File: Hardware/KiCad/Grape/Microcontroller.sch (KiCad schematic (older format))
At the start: 14 parts, among them J3 ARDUINO_R3, U4 ATMEGA328P_TQFP, Y1 16MHz

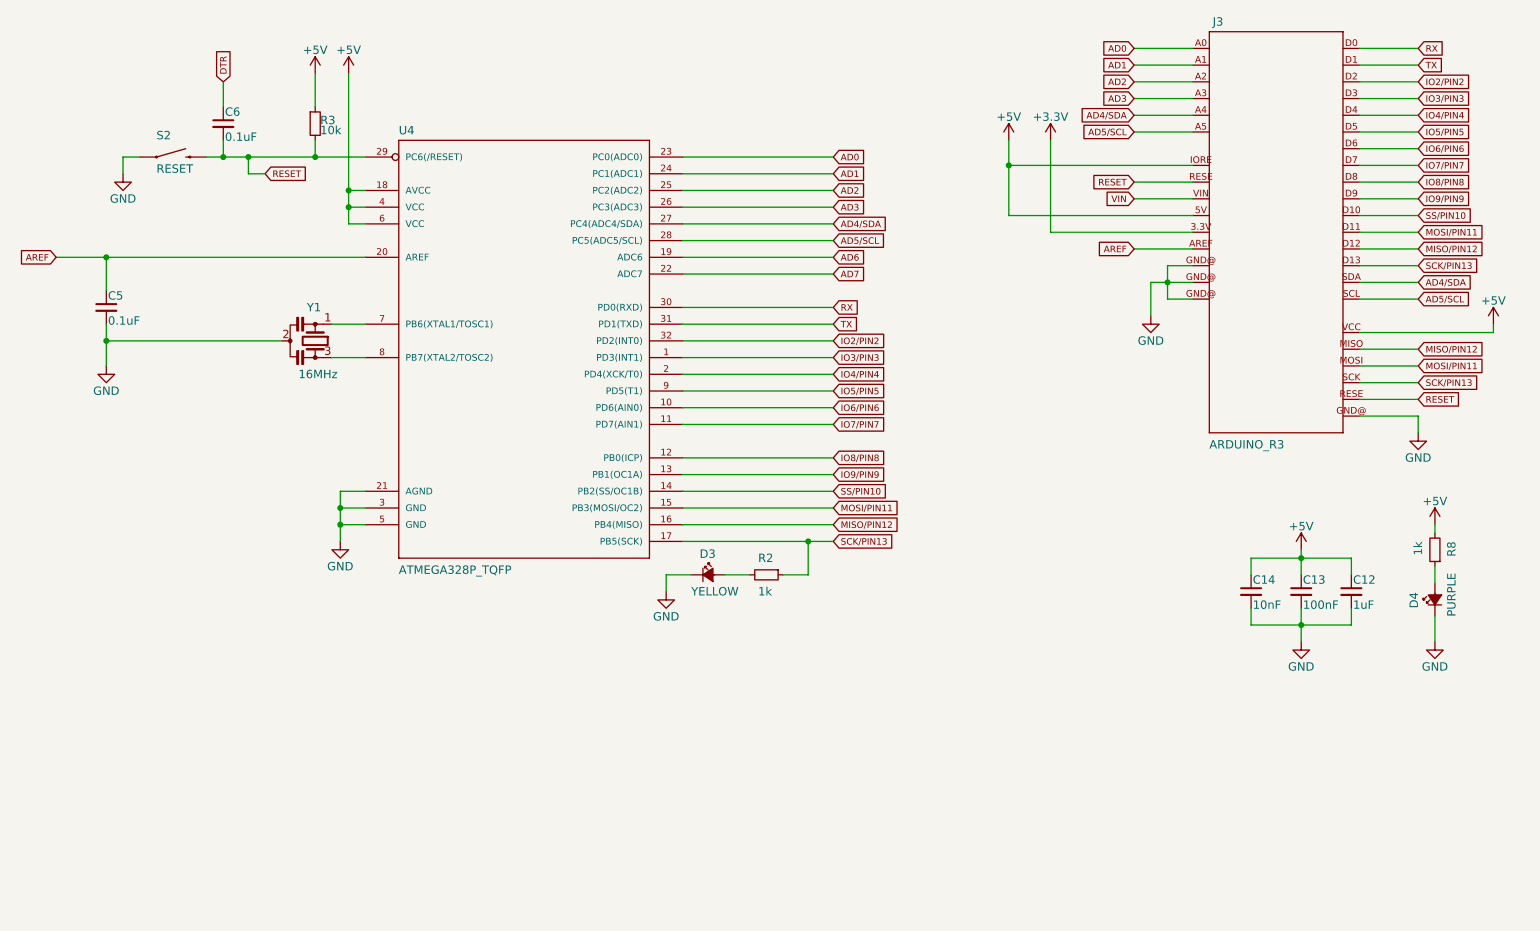
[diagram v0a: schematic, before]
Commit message: Esquema terminado y  ERC pasado
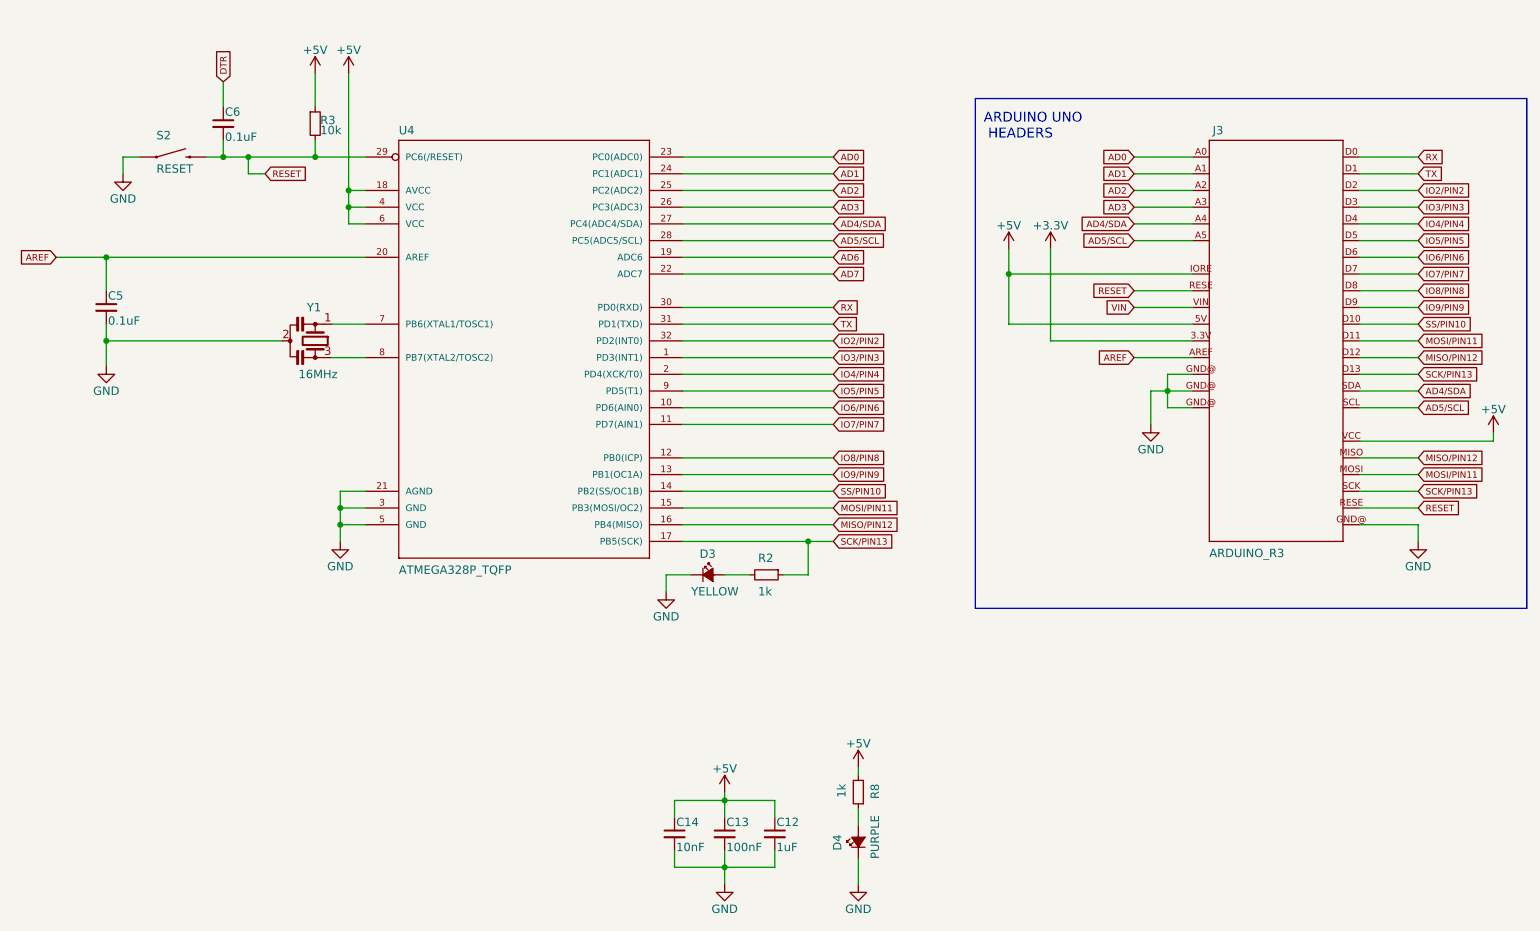
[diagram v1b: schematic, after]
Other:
- note added: "ARDUINO UNO\n HEADERS"
- moved on the sheet: C12, C13, C14, D4, J3, R8
